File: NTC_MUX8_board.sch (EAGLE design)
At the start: 62 parts, among them IC1 NINA-B306-00B-00, IC2 INA126E, IC3 MCP6001T_SOT23, IC4 MAX8559ETAAA+T, J1 USB4105-GF-A, J2 1761681-7, J3 DM3CS-SF-PEJMS, J4 DNP, Q1 NTR5103NT1G, U1 TMUX1208PWR, U2 TMUX1208PWR, U3 TMUX1208PWR, U4 TMUX1208PWR

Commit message: Pequeños errores y adición de mejoras
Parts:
- removed 5VMT1: TESTPOINT_TPS-SMD-10SN, 52101-101-REV-A_v16:TESTPOINT_TPS-SMD-10SN
- removed Q1: NTR5103NT1G, NTR5103NT1G:NTR5103NT1G
- added J7: 52808-2071, 52808-2071:52808-2071
- added SV1: (no value), con-lstb:MA03-1
- added TPSV+: TESTPOINT_TPS-SMD-10SN, 52101-101-REV-A_v16:TESTPOINT_TPS-SMD-10SN
- added X1: 22-23-2021, con-molex:22-23-2021
- renumbered 3V3T2 to 3V3T1
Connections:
- net EN1 renamed ENI1
- net EN2 renamed ENI2
- removed net 5VMOSFET: 5VMT1.TP, C12.1, Q1.S, RV1.PA0, RV1.VDD, U1.D, U1.VDD, U2.D, U2.VDD, U3.VDD, U4.VDD
- removed net EN3: IC1.GPIO_21, R6.2, U3.EN
- removed net EN4: IC1.GPIO_22, R7.2, U4.EN
- removed net MOSFET1: Q1.G
- removed net N$13: R21.1
- new net DAT: J3.DAT1, J3.DAT2, R21.1
- new net ENO1: IC1.GPIO_22, R6.2, U3.EN
- new net ENO2: IC1.GPIO_21, R7.2, U4.EN
- new net VSEL: C12.1, RV1.PA0, RV1.VDD, SV1.2, TPSV+.TP, U1.D, U1.VDD, U2.D, U2.VDD, U3.VDD, U4.VDD
- net 3V3_1: now also 3V3T1.TP
- net 3V3_2: now also SV1.3; no longer 3V3T1.TP
- net AIN0: now also IC1.QSPI_D2/GPIO_49
- net AIN1: now also IC1.GPIO_27
- net AIN2: now also IC1.GPIO_44
- net AOUT0: now also IC1.GPIO_39
- net AOUT1: now also IC1.GPIO_41
- net AOUT2: now also IC1.GPIO_43
- net C1IN: now also J2.20, J7.20, U2.S1; no longer J2.19, U1.S6
- net C1OUT: now also J2.9, J7.9, U4.S1; no longer J2.10, U3.S6
- net C2IN: now also J2.18, J7.18, U2.S2; no longer J2.17, U1.S7
- net C2OUT: now also J2.7, J7.7, U4.S2; no longer J2.8, U3.S7
- net C3IN: now also J2.16, J7.16, U2.S3; no longer J2.15, U1.S8
- net C3OUT: now also J2.5, J7.5, U4.S3; no longer J2.6, U3.S8
- net C4IN: now also J2.14, J7.14, U2.S4; no longer J2.13, U2.S1
- net C4OUT: now also J2.3, J7.3, U4.S4; no longer J2.4, U4.S1
- net C5IN: now also J2.12, J7.12, U2.S5; no longer J2.11, U2.S2
- net C5OUT: now also J2.1, J7.1, U4.S5; no longer J2.2, U4.S2
- net CS_3: now also J6.3; no longer J6.4
- net CS_4: now also J6.4; no longer J6.3
- net F1IN: now also J2.19, J7.19; no longer J2.20
- net F1OUT: now also J2.10, J7.10; no longer J2.9
- net F2IN: now also J2.17, J7.17; no longer J2.18
- net F2OUT: now also J2.8, J7.8; no longer J2.7
- net F3IN: now also J2.15, J7.15; no longer J2.16
- net F3OUT: now also J2.6, J7.6; no longer J2.5
- net F4IN: now also J2.13, J7.13; no longer J2.14
- net F4OUT: now also J2.4, J7.4; no longer J2.3
- net F5IN: now also J2.11, J7.11; no longer J2.12
- net F5OUT: now also J2.2, J7.2; no longer J2.1
- net GND: now also X1-1.S
- net GP_PB: now also IC1.GPIO_37
- net VBUS: no longer Q1.D
- net V_EN: now also IC1.QSPI_D0/GPIO_50; no longer IC1.QSPI_D2/GPIO_49
- net V_USB: now also SV1.1, X1-2.S
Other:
- note removed: "Añadir ADC ADS1220 (FUTURO)"
- note removed: "Añadir conector plano de +42 pines (FUTURO)"
- note removed: "Añadir headers para sacar i2c y spi"
- note removed: "Añadir ic para carga y descarga de baterías (FUTURO)"
- note removed: "Conectar MCU a pines"
- note removed: "Controlar la salida 2 del regulador para encender/apagar circuitos"
- note removed: "Jumper para saltar de 3.3v a 5v"
- note removed: "Revisar mosfets, se están usando como canal P y no N"
- note removed: "TO DO LIST"
- note removed: "Validar conexión spi y componentes para micro SD"
- note removed: "Validar secuencia en MUXes"
- note removed: "editar footprint de nina para quitar todos los gpio no usados"
- moved on the sheet: C12, C13, C8, C9, IC2, IC3, J2, J3, J4, J5, J6, JP1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

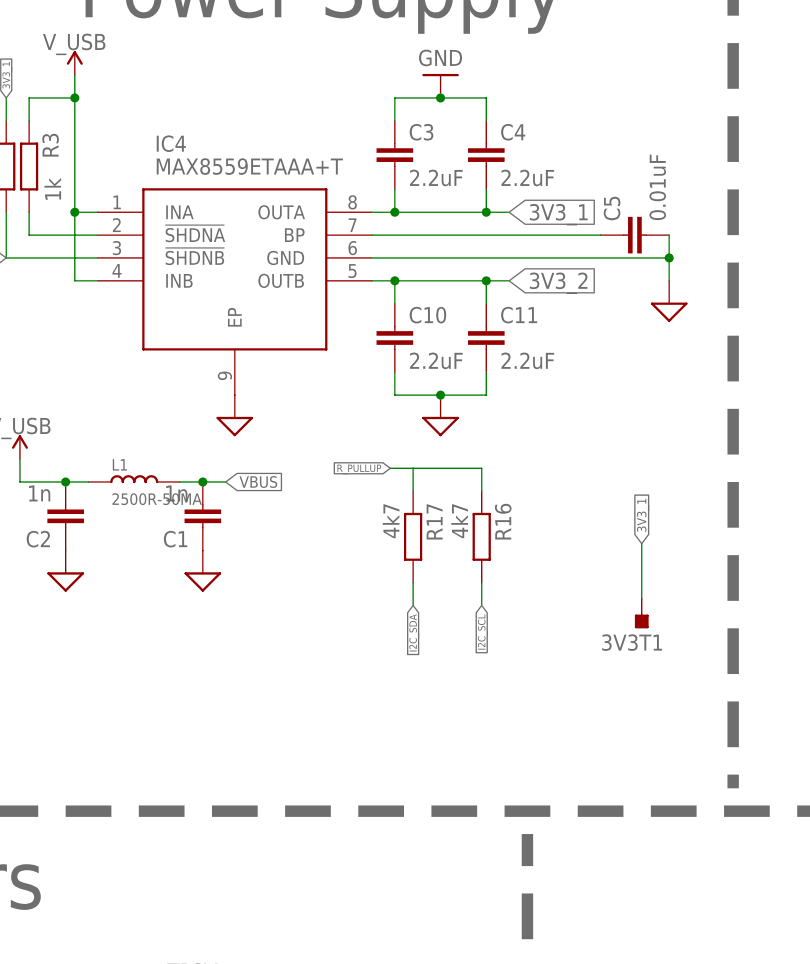
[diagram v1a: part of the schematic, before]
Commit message: beta finalizada
circuito listo a mi parecer
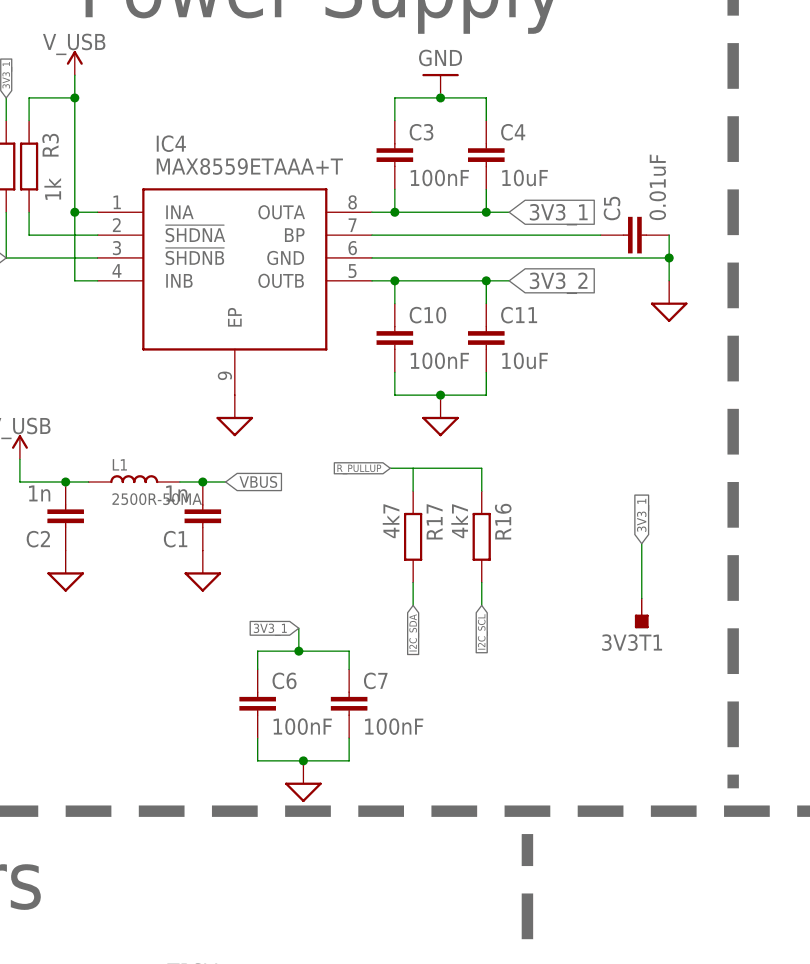
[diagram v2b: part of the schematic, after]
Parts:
- added C6, C7: 100nF, rcl:C-EUC0603
- C10, C3: value 2.2uF -> 100nF
- C11, C4: value 2.2uF -> 10uF
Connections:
- net 3V3_1: now also C6.1, C7.1
- net GND: now also C6.2, C7.2
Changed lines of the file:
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@@
 <part name="SUPPLY2" library="SparkFun-PowerSymbols" library_urn="urn:adsk.eagle:library:530" deviceset="V_USB" device=""/>
 <part name="GND5" library="audio amplifier example" library_urn="urn:adsk.eagle:library:970892" deviceset="GND" device="" value="SUP"/>
-<part name="L1" library="OPL_Ferrite_and_Magnetic_Bead" library_urn="urn:adsk.eagle:library:8004552" deviceset="SMD-FERRITE-BEAD-2500R-50MA(0603)" device="" package3d_urn="urn:adsk.eagle:package:8004622/1" value="2500R-50MA"/>
+<part name="L1" library="OPL_Ferrite_and_Magnetic_Bead" library_urn="urn:adsk.eagle:library:8004552" deviceset="SMD-FERRITE-BEAD-2500R-50MA(0603)" device="" package3d_urn="urn:adsk.eagle:package:8004622/1" override_package3d_urn="urn:adsk.eagle:package:39374540/2" override_package_urn="urn:adsk.eagle:footprint:8004597/1" value="2500R-50MA"/>
 <part name="GND6" library="audio amplifier example" library_urn="urn:adsk.eagle:library:970892" deviceset="GND" device="" value="SUP"/>
 <part name="GND7" library="audio amplifier example" library_urn="urn:adsk.eagle:library:970892" deviceset="GND" device="" value="SUP"/>
@@
 <part name="R4" library="rcl" library_urn="urn:adsk.eagle:library:334" deviceset="R-EU_" device="R0603" package3d_urn="urn:adsk.eagle:package:23555/3" value="1k"/>
 <part name="SUPPLY5" library="SparkFun-PowerSymbols" library_urn="urn:adsk.eagle:library:530" deviceset="V_USB" device=""/>
-<part name="C3" library="rcl" library_urn="urn:adsk.eagle:library:334" deviceset="C-EU" device="C0603" package3d_urn="urn:adsk.eagle:package:23616/2" value="2.2uF"/>
-<part name="C4" library="rcl" library_urn="urn:adsk.eagle:library:334" deviceset="C-EU" device="C0603" package3d_urn="urn:adsk.eagle:package:23616/2" value="2.2uF"/>
+<part name="C3" library="rcl" library_urn="urn:adsk.eagle:library:334" deviceset="C-EU" device="C0603" package3d_urn="urn:adsk.eagle:package:23616/2" value="100nF"/>
+<part name="C4" library="rcl" library_urn="urn:adsk.eagle:library:334" deviceset="C-EU" device="C0603" package3d_urn="urn:adsk.eagle:package:23616/2" value="10uF"/>
 <part name="SUPPLY24" library="Power_Symbols" library_urn="urn:adsk.eagle:library:16502351" deviceset="GND-BAR" device="" value="GND"/>
 <part name="GND10" library="audio amplifier example" library_urn="urn:adsk.eagle:library:970892" deviceset="GND" device="" value="SUP"/>
 <part name="C5" library="rcl" library_urn="urn:adsk.eagle:library:334" deviceset="C-EU" device="C0603" package3d_urn="urn:adsk.eagle:package:23616/2" value="0.01uF"/>
 <part name="GND11" library="audio amplifier example" library_urn="urn:adsk.eagle:library:970892" deviceset="GND" device="" value="SUP"/>
-<part name="C10" library="rcl" library_urn="urn:adsk.eagle:library:334" deviceset="C-EU" device="C0603" package3d_urn="urn:adsk.eagle:package:23616/2" value="2.2uF"/>
-<part name="C11" library="rcl" library_urn="urn:adsk.eagle:library:334" deviceset="C-EU" device="C0603" package3d_urn="urn:adsk.eagle:package:23616/2" value="2.2uF"/>
+<part name="C10" library="rcl" library_urn="urn:adsk.eagle:library:334" deviceset="C-EU" device="C0603" package3d_urn="urn:adsk.eagle:package:23616/2" value="100nF"/>
+<part name="C11" library="rcl" library_urn="urn:adsk.eagle:library:334" deviceset="C-EU" device="C0603" package3d_urn="urn:adsk.eagle:package:23616/2" value="10uF"/>
 <part name="GND12" library="audio amplifier example" library_urn="urn:adsk.eagle:library:970892" deviceset="GND" device="" value="SUP"/>
 <part name="U1" library="TMUX1208" deviceset="TMUX1208PWR" device="" override_package3d_urn="urn:adsk.eagle:package:39256706/3" override_package_urn="urn:adsk.eagle:footprint:39256707/1"/>
@@
 <part name="JP1" library="SparkFun-Jumpers" library_urn="urn:adsk.eagle:library:528" deviceset="JUMPER-SMT_3_NO" device="_NO-SILK" package3d_urn="urn:adsk.eagle:package:39284/1" override_package3d_urn="urn:adsk.eagle:package:39329052/2" override_package_urn="urn:adsk.eagle:footprint:39263/1"/>
 <part name="GND32" library="Arduino-supply" deviceset="GND" device="" value="GND"/>
-<part name="D2" library="SML-P12PTT86R" deviceset="SML-P12PTT86R" device="" override_package3d_urn="urn:adsk.eagle:package:39329460/2" override_package_urn="urn:adsk.eagle:footprint:39329461/1"/>
+<part name="D2" library="SML-P12PTT86R" deviceset="SML-P12PTT86R" device="" override_package3d_urn="urn:adsk.eagle:package:39374574/2" override_package_urn="urn:adsk.eagle:footprint:39374575/1"/>
 <part name="J6" library="con-lstb" library_urn="urn:adsk.eagle:library:162" deviceset="MA06-2" device="" package3d_urn="urn:adsk.eagle:package:8342/1" override_package3d_urn="urn:adsk.eagle:package:39329735/3" override_package_urn="urn:adsk.eagle:footprint:8289/1"/>
 <part name="J5" library="con-lstb" library_urn="urn:adsk.eagle:library:162" deviceset="MA04-2" device="" package3d_urn="urn:adsk.eagle:package:8368/1" override_package3d_urn="urn:adsk.eagle:package:39329712/4" override_package_urn="urn:adsk.eagle:footprint:8328/1"/>
@@
 <part name="R20" library="rcl" library_urn="urn:adsk.eagle:library:334" deviceset="R-EU_" device="R0603" package3d_urn="urn:adsk.eagle:package:23555/3" value="10k"/>
 <part name="R21" library="rcl" library_urn="urn:adsk.eagle:library:334" deviceset="R-EU_" device="R0603" package3d_urn="urn:adsk.eagle:package:23555/3" value="10k"/>
-<part name="R13" library="rcl" library_urn="urn:adsk.eagle:library:334" deviceset="R-EU_" device="R0603" package3d_urn="urn:adsk.eagle:package:23555/3" value="DNP"/>
-<part name="R14" library="rcl" library_urn="urn:adsk.eagle:library:334" deviceset="R-EU_" device="R0603" package3d_urn="urn:adsk.eagle:package:23555/3" value="DNP"/>
+<part name="R13" library="rcl" library_urn="urn:adsk.eagle:library:334" deviceset="R-EU_" device="R0603" package3d_urn="urn:adsk.eagle:package:23555/3" override_package3d_urn="urn:adsk.eagle:package:39374572/2" override_package_urn="urn:adsk.eagle:footprint:23044/1" value="DNP"/>
+<part name="R14" library="rcl" library_urn="urn:adsk.eagle:library:334" deviceset="R-EU_" device="R0603" package3d_urn="urn:adsk.eagle:package:23555/3" override_package3d_urn="urn:adsk.eagle:package:39374573/2" override_package_urn="urn:adsk.eagle:footprint:23044/1" value="DNP"/>
 <part name="SV1" library="con-lstb" library_urn="urn:adsk.eagle:library:162" deviceset="MA03-1" device="" package3d_urn="urn:adsk.eagle:package:8339/1" override_package3d_urn="urn:adsk.eagle:package:39362152/2" override_package_urn="urn:adsk.eagle:footprint:8281/1"/>
 <part name="X1" library="con-molex" library_urn="urn:adsk.eagle:library:165" deviceset="22-23-2021" device="" package3d_urn="urn:adsk.eagle:package:8078633/1" override_package3d_urn="urn:adsk.eagle:package:39362140/2" override_package_urn="urn:adsk.eagle:footprint:8078259/1"/>
 <part name="J7" library="52808-2071" deviceset="52808-2071" device="" override_package3d_urn="urn:adsk.eagle:package:39362400/2" override_package_urn="urn:adsk.eagle:footprint:39362401/1"/>
+<part name="C6" library="rcl" library_urn="urn:adsk.eagle:library:334" deviceset="C-EU" device="C0603" package3d_urn="urn:adsk.eagle:package:23616/2" override_package3d_urn="urn:adsk.eagle:package:39374531/2" override_package_urn="urn:adsk.eagle:footprint:23123/1" value="100nF"/>
+<part name="C7" library="rcl" library_urn="urn:adsk.eagle:library:334" deviceset="C-EU" device="C0603" package3d_urn="urn:adsk.eagle:package:23616/2" override_package3d_urn="urn:adsk.eagle:package:39374516/2" override_package_urn="urn:adsk.eagle:footprint:23123/1" value="100nF"/>
+<part name="GND9" library="audio amplifier example" library_urn="urn:adsk.eagle:library:970892" deviceset="GND" device="" value="SUP"/>
 </parts>
 <sheets>
@@
 <attribute name="VALUE" x="105.41" y="58.42" size="1.778" layer="96" align="center-left"/>
 </instance>
+<instance part="C6" gate="G$1" x="140.208" y="168.148" smashed="yes">
+<attribute name="NAME" x="141.732" y="168.529" size="1.778" layer="95"/>
+<attribute name="VALUE" x="141.732" y="163.449" size="1.778" layer="96"/>
+</instance>
+<instance part="C7" gate="G$1" x="150.368" y="168.148" smashed="yes">
+<attribute name="NAME" x="151.892" y="168.529" size="1.778" layer="95"/>
+<attribute name="VALUE" x="151.892" y="163.449" size="1.778" layer="96"/>
+</instance>
+<instance part="GND9" gate="G$1" x="145.288" y="160.528" smashed="yes"/>
 </instances>
 <busses>
@@
 <label x="157.48" y="132.08" size="1.016" layer="95" xref="yes"/>
 </segment>
+<segment>
+<pinref part="C6" gate="G$1" pin="2"/>
+<wire x1="140.208" y1="163.068" x2="140.208" y2="160.528" width="0.1524" layer="91"/>
+<wire x1="140.208" y1="160.528" x2="145.288" y2="160.528" width="0.1524" layer="91"/>
+<pinref part="C7" gate="G$1" pin="2"/>
+<wire x1="145.288" y1="160.528" x2="150.368" y2="160.528" width="0.1524" layer="91"/>
+<wire x1="150.368" y1="160.528" x2="150.368" y2="163.068" width="0.1524" layer="91"/>
+<pinref part="GND9" gate="G$1" pin="GND"/>
+<junction x="145.288" y="160.528"/>
+</segment>
 </net>
 <net name="N$1" class="0">
@@
 <pinref part="3V3T1" gate="G$1" pin="TP"/>
 </segment>
+<segment>
+<pinref part="C6" gate="G$1" pin="1"/>
+<wire x1="140.208" y1="170.688" x2="140.208" y2="172.72" width="0.1524" layer="91"/>
+<wire x1="140.208" y1="172.72" x2="144.78" y2="172.72" width="0.1524" layer="91"/>
+<pinref part="C7" gate="G$1" pin="1"/>
+<wire x1="144.78" y1="172.72" x2="150.368" y2="172.72" width="0.1524" layer="91"/>
+<wire x1="150.368" y1="172.72" x2="150.368" y2="170.688" width="0.1524" layer="91"/>
+<wire x1="144.78" y1="172.72" x2="144.78" y2="175.26" width="0.1524" layer="91"/>
+<junction x="144.78" y="172.72"/>
+<label x="144.78" y="175.26" size="1.016" layer="95" rot="R180" xref="yes"/>
+</segment>
 </net>
